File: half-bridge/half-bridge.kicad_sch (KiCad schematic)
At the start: 61 parts, among them J1 Conn_01x11_Pin, J2 Conn_01x11_Pin, J3 Conn_01x04_Pin, J4 Conn_01x04_Pin, J5 Conn_01x11_Pin, J6 Conn_01x11_Pin, J7 Conn_01x11_Pin, J8 Conn_01x11_Pin, Q1 GAN7R0-150LBE, Q2 GAN7R0-150LBE, U1 LMG1210

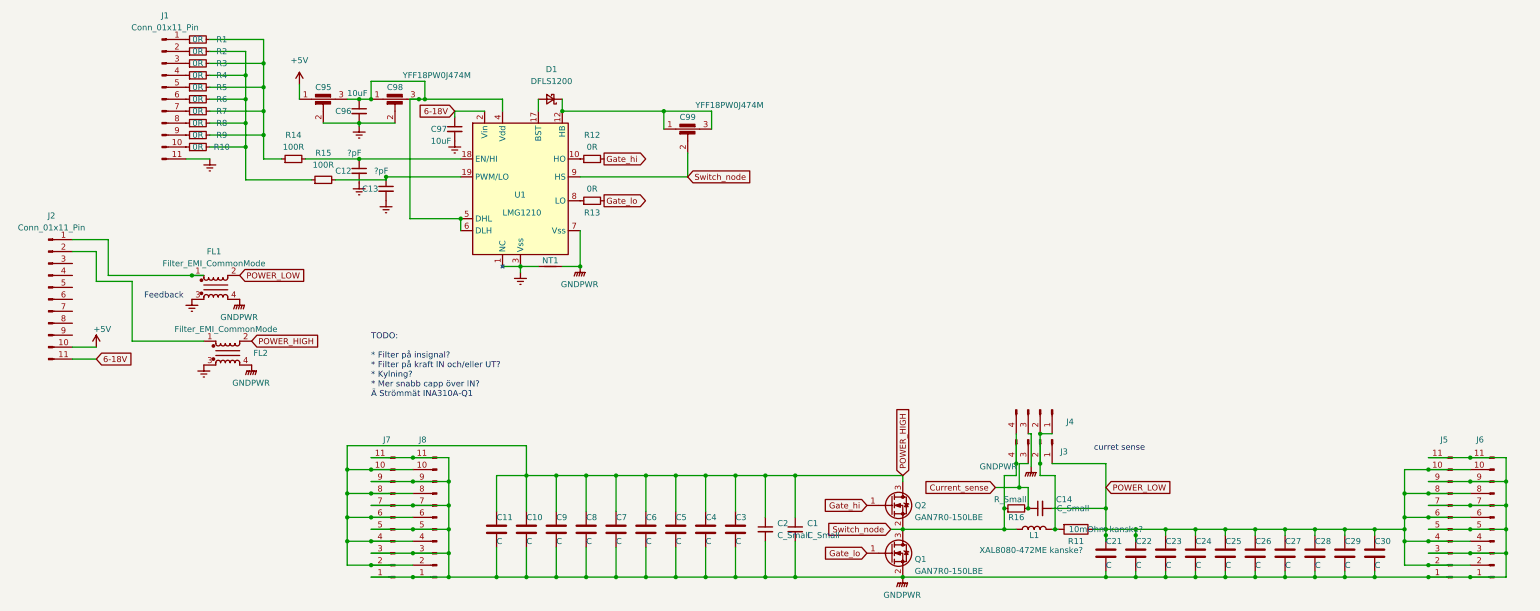
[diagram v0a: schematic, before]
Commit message: More work on current sense
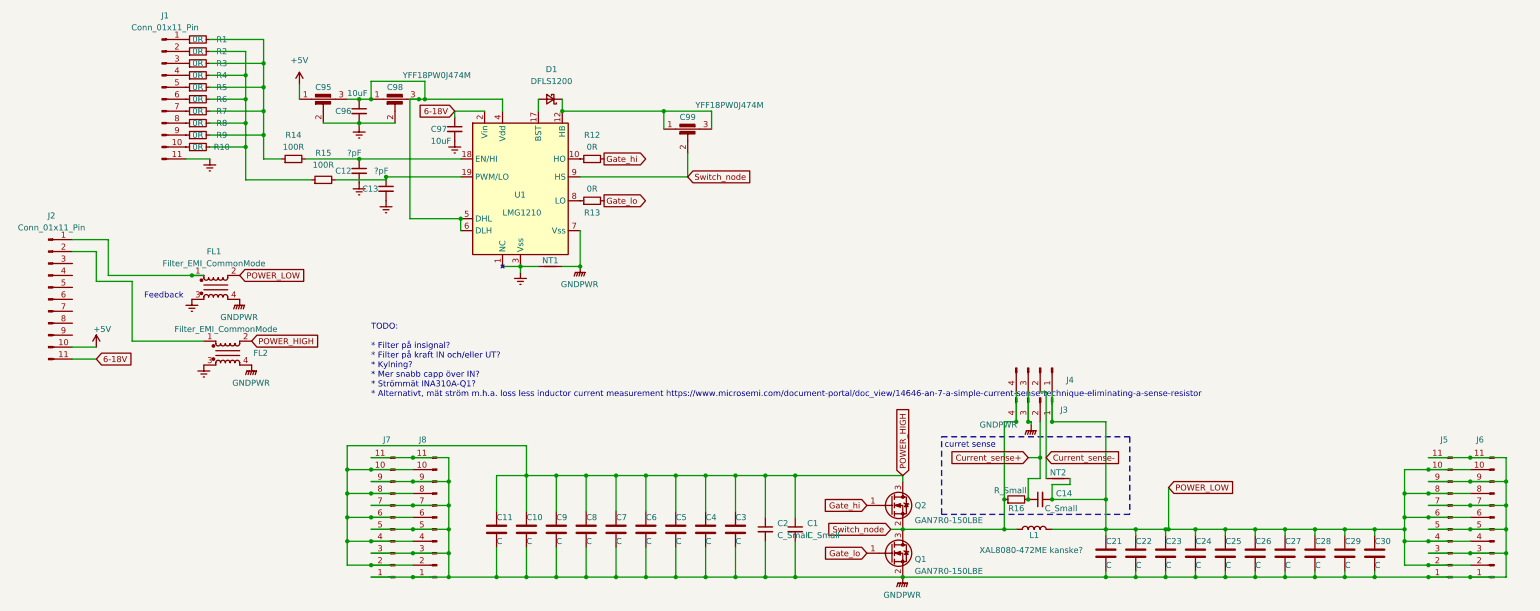
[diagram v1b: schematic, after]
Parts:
- removed R11: 10mOhm kanske?, Resistor_SMD:R_2816_7142Metric, symbol Device:R
- added NT2: NetTie_2, NetTie:NetTie-2_SMD_Pad0.5mm, symbol Device:NetTie_2
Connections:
- net GNDPWR: now also J3.3 (Pin_3)
- net POWER_LOW: now also J4.1 (Pin_1), L1.2, NT2.2
- net Current_sense renamed Current_sense+
- net Current_sense+: now also J3.2 (Pin_2); no longer J3.3 (Pin_3)
- new net Current_sense-: J4.2 (Pin_2), NT2.1
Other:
- note added: "TODO: * Filter på insignal? * Filter på kraft IN och/eller UT? * Kylning? * Mer snabb capp över IN? * Strömmät INA310A-Q1? * Alternativt, mät ström m.h.a. loss less inductor current measurement https://www.microsemi.com/document-portal/doc_view/14646-an-7-a-simple-current-sense-technique-eliminating-a-sense-resistor"
- note removed: "TODO: * Filter på insignal? * Filter på kraft IN och/eller UT? * Kylning? * Mer snabb capp över IN? Ä Strömmät INA310A-Q1"
- moved on the sheet: C14, J3, J4, R16
